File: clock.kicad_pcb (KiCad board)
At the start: 4 copper layers, 32 x 30 mm, 30 parts, among them J1 CONN_01X05, P1 USB_OTG, P2 CONN_01X02, U1 oled_i2c_display_128x64, U2 FM24V10-G, U3 STLCS01V1, U4 mcp73831, U5 lmv341, U6 NCP170

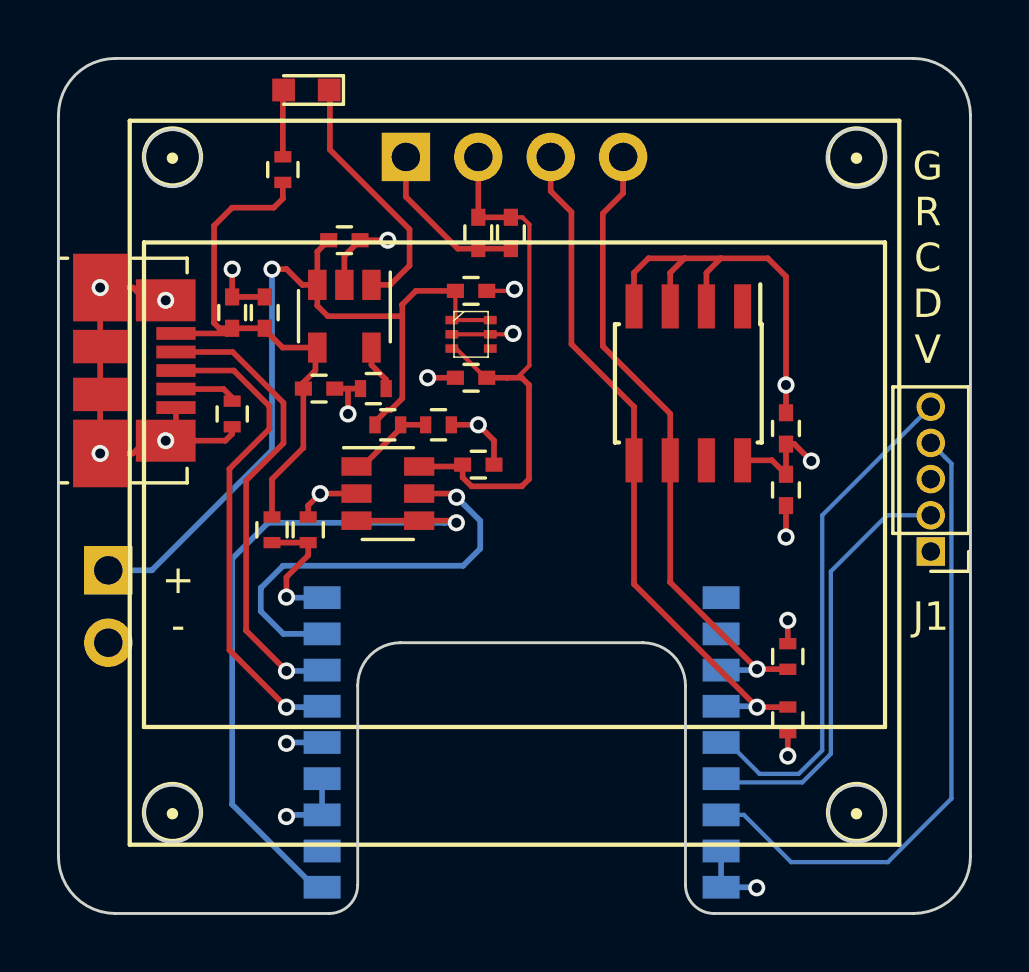
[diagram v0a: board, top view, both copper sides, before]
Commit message: small modif
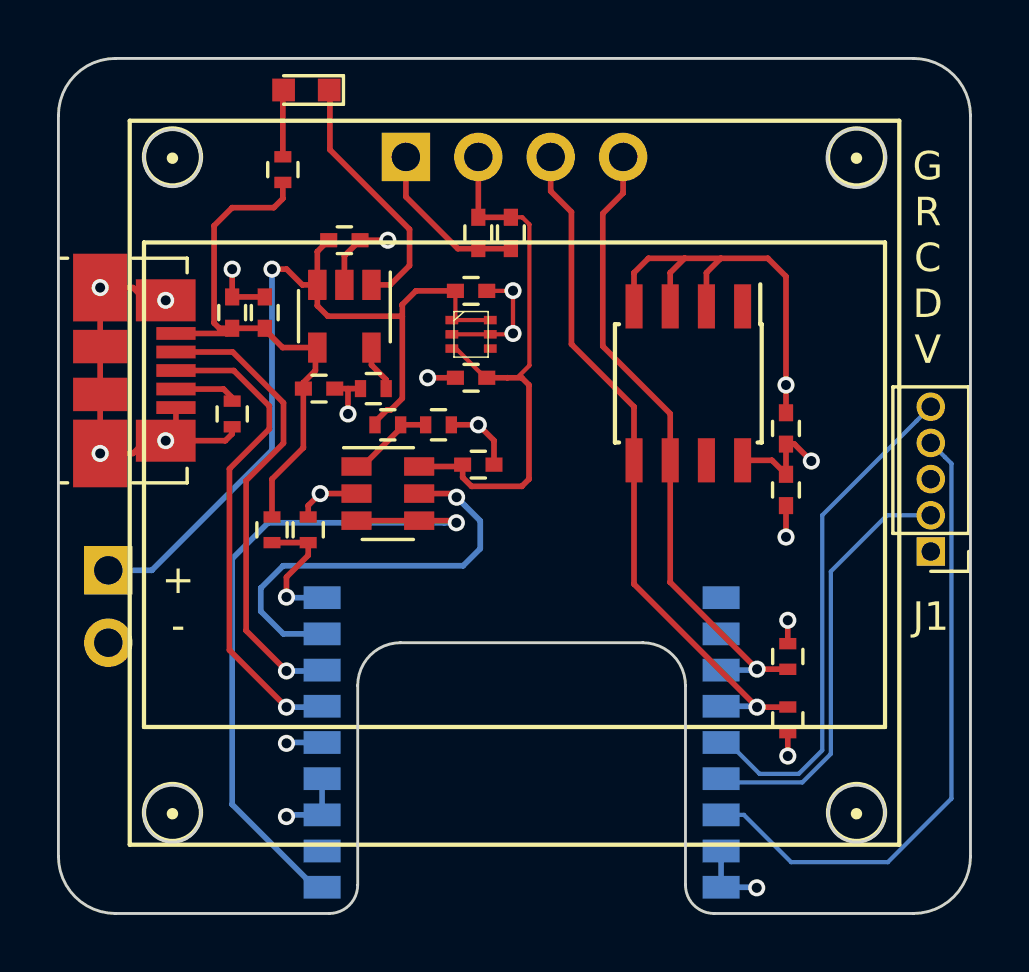
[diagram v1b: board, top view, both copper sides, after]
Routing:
- net GND: track 56.7 -> 58.1 mm
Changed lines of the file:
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@@
   (general
     (links 82)
-    (no_connects 5)
+    (no_connects 0)
     (area 149.949999 69.949999 182.050001 100.050001)
     (thickness 1.6)
     (drawings 30)
-    (tracks 265)
+    (tracks 266)
     (zones 0)
     (modules 30)
@@
   (gr_line (start 152 70) (end 180 70) (layer Edge.Cuts) (width 0.1))
   (gr_line (start 150 98) (end 150 72) (layer Edge.Cuts) (width 0.1))
+  (segment (start 165.95 78.15) (end 165.95 79.65) (width 0.15) (layer F.Cu) (net 1))
+  (segment (start 165.028 78.156) (end 165.944 78.156) (width 0.15) (layer F.Cu) (net 1))
+  (segment (start 165.944 78.156) (end 165.95 78.15) (width 0.15) (layer F.Cu) (net 1))
+  (via (at 165.95 78.15) (size 0.6) (drill 0.35) (layers F.Cu B.Cu) (net 1))
   (segment (start 165.92 79.68) (end 165.95 79.65) (width 0.15) (layer F.Cu) (net 1))
   (segment (start 165.153 79.68) (end 165.92 79.68) (width 0.15) (layer F.Cu) (net 1))
   (via (at 165.95 79.65) (size 0.6) (drill 0.35) (layers F.Cu B.Cu) (net 1))
-  (segment (start 165.028 78.156) (end 165.944 78.156) (width 0.15) (layer F.Cu) (net 1))
-  (via (at 166 78.1) (size 0.6) (drill 0.35) (layers F.Cu B.Cu) (net 1))
-  (segment (start 165.944 78.156) (end 166 78.1) (width 0.15) (layer F.Cu) (net 1))
   (segment (start 163.803 79.68) (end 165.153 79.68) (width 0.15) (layer F.Cu) (net 1))
   (segment (start 174.48 99.08) (end 174.5 99.1) (width 0.2) (layer B.Cu) (net 1))
